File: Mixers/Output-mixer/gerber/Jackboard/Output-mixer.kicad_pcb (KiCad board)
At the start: 2 copper layers, 135 x 110 mm, 131 parts, among them J1 In, J10 In, J11 In, J12 In, J14 Conn_01x04_Female, J17 Conn_01x02_Female, J2 In, J21 Jack 3.5 Out, J22 OutL, J23 OutR, J25 Conn_01x02_Female, J3 In, J4 In, J5 In, J6 In, J7 In, J8 In, J9 In, Q10 2N3904, Q5 2N3904, Q6 2N3904, Q7 2N3904, Q8 2N3904, Q9 2N3904, SW1 Mute, SW2 Mute, SW3 Mute, SW4 Mute, SW5 Mute, SW6 Mute, U1 TL072, U2 TL072, U3 TL072

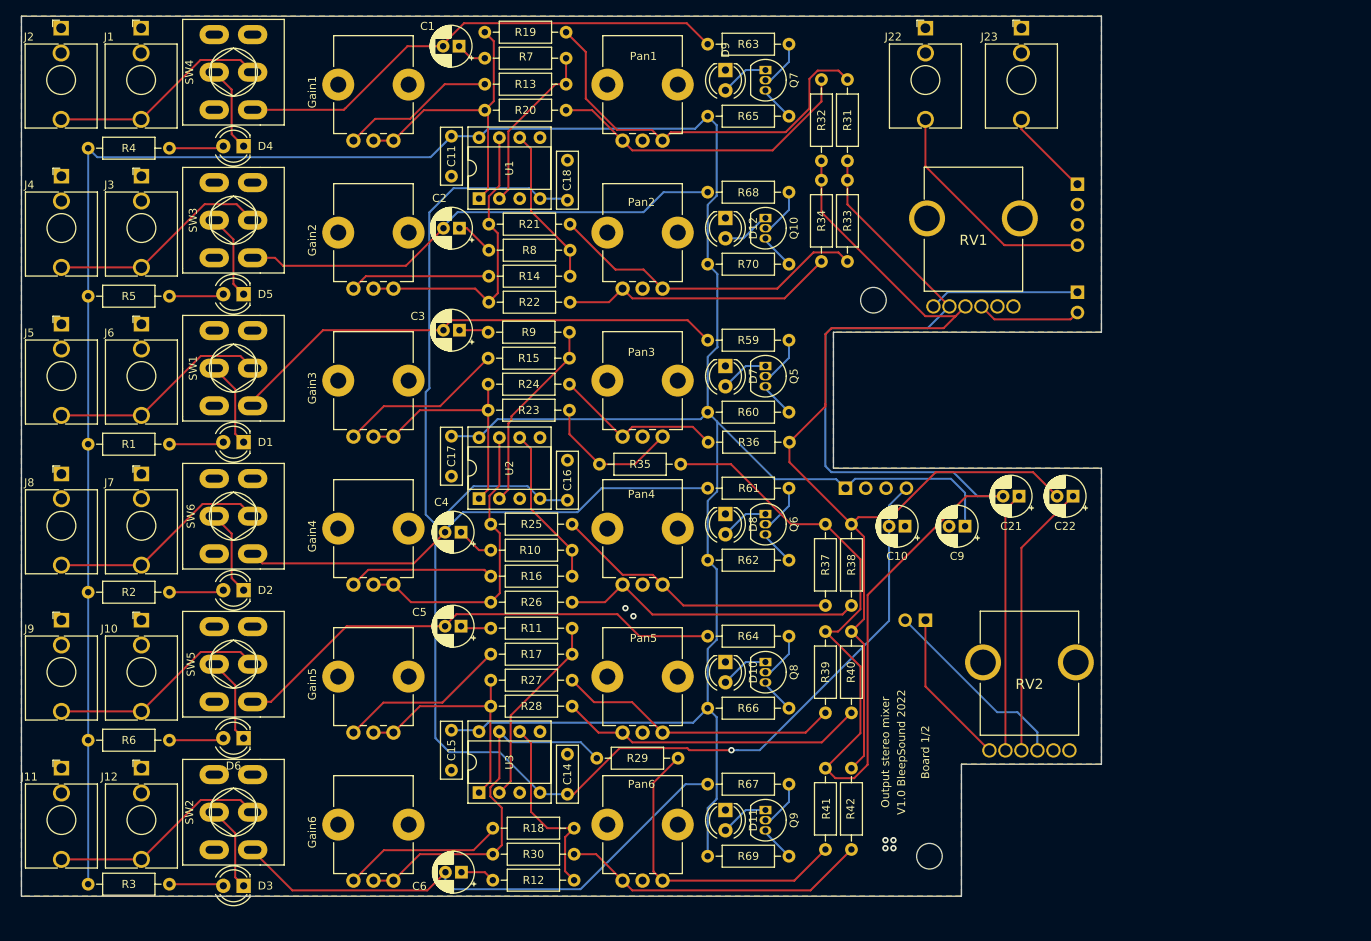
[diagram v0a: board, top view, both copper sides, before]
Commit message: quick update
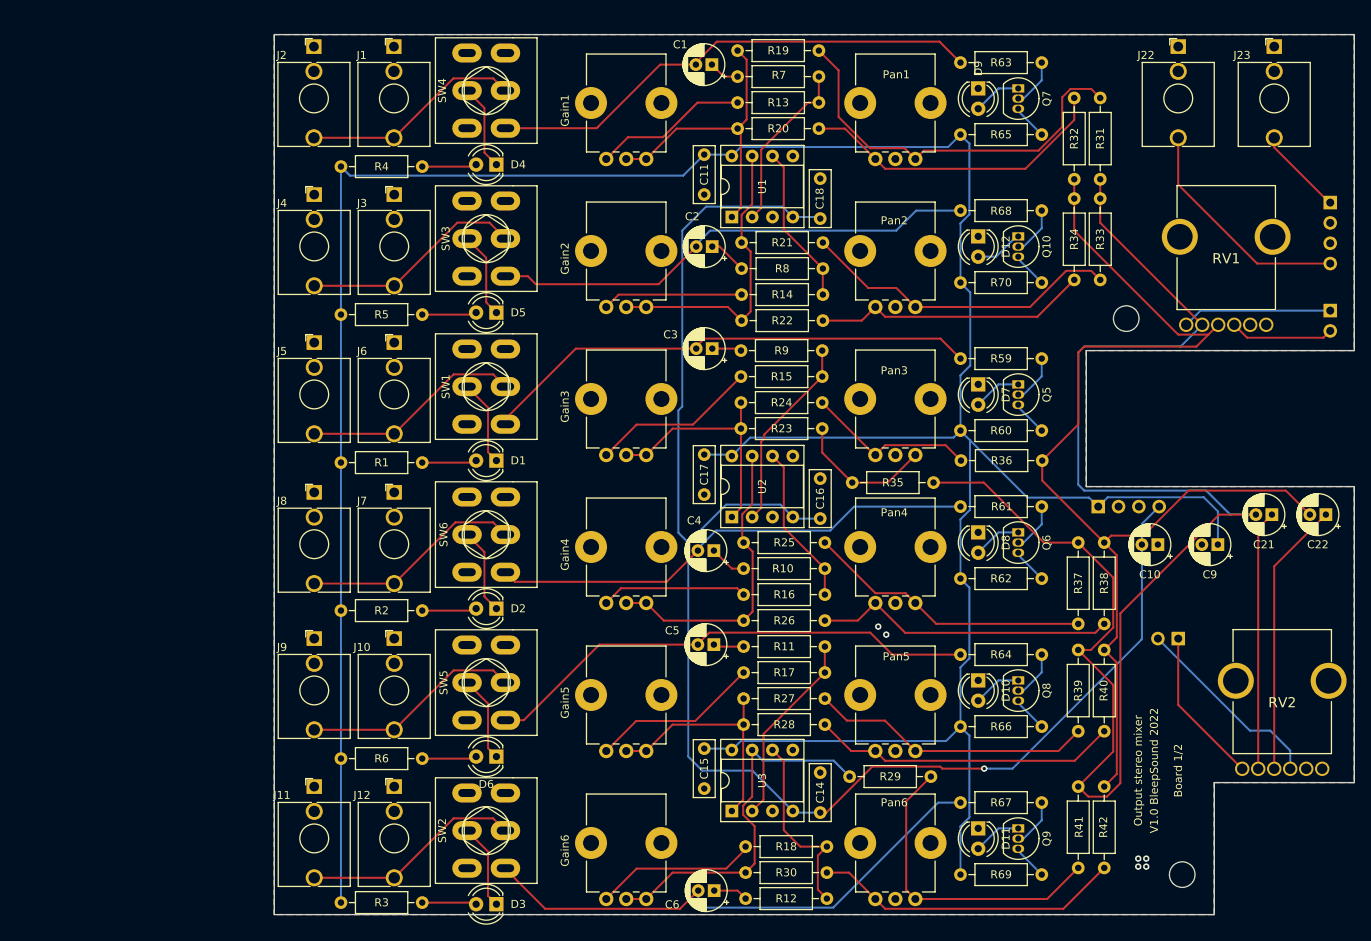
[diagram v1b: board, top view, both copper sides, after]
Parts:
- moved C1 31.7 mm to (103.3, 37.0)
- moved C10 31.7 mm to (159.1, 97.0)
- moved Pan1 31.7 mm to (128.7, 48.9)
- moved Pan2 31.7 mm to (128.7, 67.3)
- moved Pan3 31.7 mm to (128.7, 85.8)
- moved Pan4 31.7 mm to (128.7, 104.3)
- moved Pan5 31.7 mm to (128.7, 122.8)
- moved R10 31.7 mm to (117.4, 100.0)
- moved R11 31.7 mm to (117.4, 109.8)
- moved R12 31.7 mm to (117.7, 141.3)
- moved R20 31.7 mm to (116.7, 45.0)
- moved R22 31.7 mm to (117.2, 69.0)
- moved R26 31.7 mm to (117.4, 106.5)
- moved R28 31.7 mm to (117.4, 119.5)
- moved R30 31.7 mm to (117.7, 138.1)
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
